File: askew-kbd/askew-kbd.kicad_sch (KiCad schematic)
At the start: 57 parts, among them J1 OLED, J2 MJ-4PP-9, SW1 SW_PUSH, SW10 SW_PUSH, SW11 SW_PUSH, SW12 SW_PUSH, SW13 SW_PUSH, SW14 SW_PUSH, SW15 SW_PUSH, SW16 SW_PUSH, SW17 SW_PUSH, SW18 SW_PUSH, SW19 SW_PUSH, SW2 SW_PUSH, SW20 SW_PUSH, SW21 SW_PUSH, SW22 SW_PUSH, SW3 SW_PUSH, SW4 SW_PUSH, SW5 SW_PUSH, SW6 SW_PUSH, SW7 SW_PUSH, SW8 SW_PUSH, SW9 SW_PUSH, U1 ProMicro

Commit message: choc_spacing
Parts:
- SW1, SW10, SW11, SW12, SW13, SW14, SW15, SW16, SW17, SW18, SW2, SW21, SW3, SW4, SW5, SW6, SW7, SW8, SW9: footprint fp:ChocV1_V2_Hotswap_reversed -> fp:ChocV1_V2_Hotswap_reversed_choc_spacing
- SW19, SW20, SW22: footprint fp:ChocV1_V2_Hotswap_reversed_15u -> fp:ChocV1_V2_Hotswap_reversed_15u_choc_spacing

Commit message: redo layout
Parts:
- D1, D10, D11, D12, D13, D14, D15, D16, D17, D18, D19, D2, D20, D21, D22, D3, D4, D5, D6, D7, D8, D9: footprint fp:D3_SMD -> kbd:D3_TH_SMD

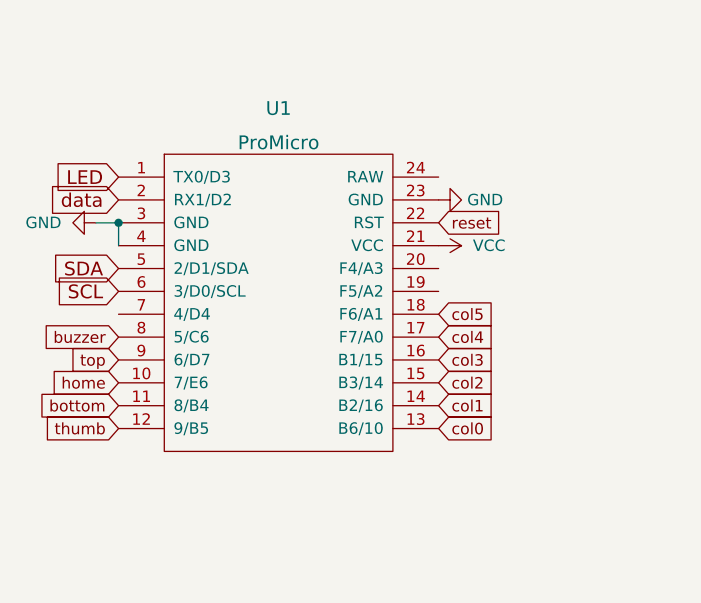
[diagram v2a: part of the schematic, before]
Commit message: basic routing
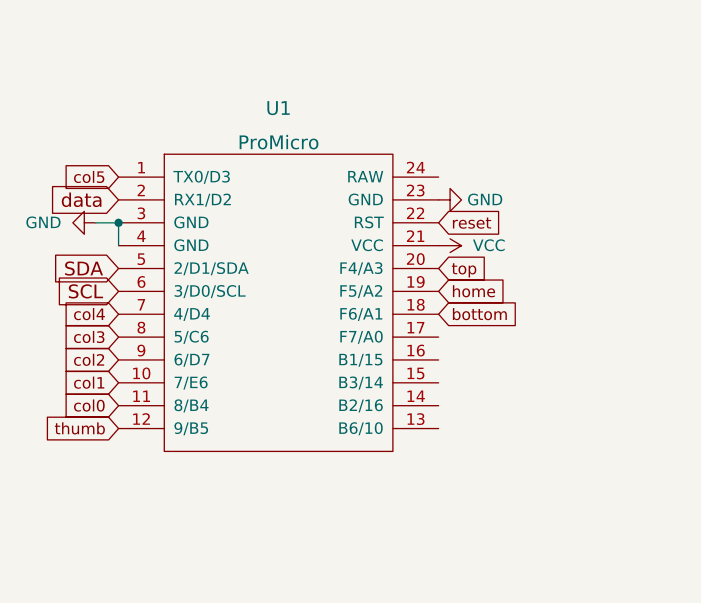
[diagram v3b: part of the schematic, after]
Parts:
- U1: footprint keyboard_reversible:ProMicro_unrouted -> fp:ProMicro_unrouted_type_c
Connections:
- net LED is gone; now on net col5: U1.1 (TX0/D3)
- net buzzer is gone; now on net col3: U1.8 (5/C6)
- net bottom: now also U1.18 (F6/A1); no longer U1.11 (8/B4)
- net col0: now also U1.11 (8/B4); no longer U1.13 (B6/10)
- net col1: now also U1.10 (7/E6); no longer U1.14 (B2/16)
- net col2: now also U1.9 (6/D7); no longer U1.15 (B3/14)
- net col3: no longer U1.16 (B1/15)
- net col4: now also U1.7 (4/D4); no longer U1.17 (F7/A0)
- net col5: no longer U1.18 (F6/A1)
- net home: now also U1.19 (F5/A2); no longer U1.10 (7/E6)
- net top: now also U1.20 (F4/A3); no longer U1.9 (6/D7)
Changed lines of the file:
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@@
     )
   )
-  (global_label "col0" (shape input) (at 91.44 74.93 0) (fields_autoplaced)
-    (effects (font (size 1.27 1.27)) (justify left))
-    (property "Intersheet References" "${INTERSHEET_REFS}" (id 0) (at 97.9655 74.8506 0)
-      (effects (font (size 1.27 1.27)) (justify left) hide)
+  (global_label "col0" (shape input) (at 55.88 72.39 180) (fields_autoplaced)
+    (effects (font (size 1.27 1.27)) (justify right))
+    (property "Intersheet References" "${INTERSHEET_REFS}" (id 0) (at 49.3545 72.4694 0)
+      (effects (font (size 1.27 1.27)) (justify right) hide)
     )
   )
@@
     )
   )
-  (global_label "bottom" (shape input) (at 55.88 72.39 180) (fields_autoplaced)
-    (effects (font (size 1.27 1.27)) (justify right))
-    (property "Intersheet References" "${INTERSHEET_REFS}" (id 0) (at 46.875 72.3106 0)
-      (effects (font (size 1.27 1.27)) (justify right) hide)
+  (global_label "bottom" (shape input) (at 91.44 62.23 0) (fields_autoplaced)
+    (effects (font (size 1.27 1.27)) (justify left))
+    (property "Intersheet References" "${INTERSHEET_REFS}" (id 0) (at 100.445 62.3094 0)
+      (effects (font (size 1.27 1.27)) (justify left) hide)
     )
   )
@@
     )
   )
-  (global_label "col5" (shape input) (at 91.44 62.23 0) (fields_autoplaced)
-    (effects (font (size 1.27 1.27)) (justify left))
-    (property "Intersheet References" "${INTERSHEET_REFS}" (id 0) (at 97.9655 62.1506 0)
-      (effects (font (size 1.27 1.27)) (justify left) hide)
+  (global_label "col5" (shape input) (at 55.88 46.99 180) (fields_autoplaced)
+    (effects (font (size 1.27 1.27)) (justify right))
+    (property "Intersheet References" "${INTERSHEET_REFS}" (id 0) (at 49.3545 47.0694 0)
+      (effects (font (size 1.27 1.27)) (justify right) hide)
     )
   )
@@
     )
   )
-  (global_label "LED" (shape input) (at 55.88 46.99 180) (fields_autoplaced)
-    (effects (font (size 1.524 1.524)) (justify right))
-    (property "Intersheet References" "${INTERSHEET_REFS}" (id 0) (at 264.795 142.875 0)
-      (effects (font (size 1.27 1.27)) hide)
-    )
-  )
-  (global_label "col3" (shape input) (at 91.44 67.31 0) (fields_autoplaced)
-    (effects (font (size 1.27 1.27)) (justify left))
-    (property "Intersheet References" "${INTERSHEET_REFS}" (id 0) (at 97.9655 67.2306 0)
-      (effects (font (size 1.27 1.27)) (justify left) hide)
+  (global_label "col3" (shape input) (at 55.88 64.77 180) (fields_autoplaced)
+    (effects (font (size 1.27 1.27)) (justify right))
+    (property "Intersheet References" "${INTERSHEET_REFS}" (id 0) (at 49.3545 64.8494 0)
+      (effects (font (size 1.27 1.27)) (justify right) hide)
     )
   )
@@
     )
   )
-  (global_label "col1" (shape input) (at 91.44 72.39 0) (fields_autoplaced)
-    (effects (font (size 1.27 1.27)) (justify left))
-    (property "Intersheet References" "${INTERSHEET_REFS}" (id 0) (at 97.9655 72.3106 0)
-      (effects (font (size 1.27 1.27)) (justify left) hide)
-    )
-  )
-  (global_label "buzzer" (shape input) (at 55.88 64.77 180) (fields_autoplaced)
+  (global_label "col1" (shape input) (at 55.88 69.85 180) (fields_autoplaced)
     (effects (font (size 1.27 1.27)) (justify right))
-    (property "Intersheet References" "${INTERSHEET_REFS}" (id 0) (at 47.2379 64.6906 0)
+    (property "Intersheet References" "${INTERSHEET_REFS}" (id 0) (at 49.3545 69.9294 0)
       (effects (font (size 1.27 1.27)) (justify right) hide)
     )
@@
     )
   )
-  (global_label "col2" (shape input) (at 91.44 69.85 0) (fields_autoplaced)
+  (global_label "col2" (shape input) (at 55.88 67.31 180) (fields_autoplaced)
+    (effects (font (size 1.27 1.27)) (justify right))
+    (property "Intersheet References" "${INTERSHEET_REFS}" (id 0) (at 49.3545 67.3894 0)
+      (effects (font (size 1.27 1.27)) (justify right) hide)
+    )
+  )
+  (global_label "home" (shape input) (at 91.44 59.69 0) (fields_autoplaced)
     (effects (font (size 1.27 1.27)) (justify left))
-    (property "Intersheet References" "${INTERSHEET_REFS}" (id 0) (at 97.9655 69.7706 0)
-      (effects (font (size 1.27 1.27)) (justify left) hide)
-    )
-  )
-  (global_label "home" (shape input) (at 55.88 69.85 180) (fields_autoplaced)
-    (effects (font (size 1.27 1.27)) (justify right))
-    (property "Intersheet References" "${INTERSHEET_REFS}" (id 0) (at 48.3869 69.7706 0)
-      (effects (font (size 1.27 1.27)) (justify right) hide)
+    (property "Intersheet References" "${INTERSHEET_REFS}" (id 0) (at 98.9331 59.7694 0)
+      (effects (font (size 1.27 1.27)) (justify left) hide)
     )
   )
@@
     )
   )
-  (global_label "top" (shape input) (at 55.88 67.31 180) (fields_autoplaced)
+  (global_label "top" (shape input) (at 91.44 57.15 0) (fields_autoplaced)
+    (effects (font (size 1.27 1.27)) (justify left))
+    (property "Intersheet References" "${INTERSHEET_REFS}" (id 0) (at 96.8769 57.2294 0)
+      (effects (font (size 1.27 1.27)) (justify left) hide)
+    )
+  )
+  (global_label "col4" (shape input) (at 55.88 62.23 180) (fields_autoplaced)
     (effects (font (size 1.27 1.27)) (justify right))
-    (property "Intersheet References" "${INTERSHEET_REFS}" (id 0) (at 50.4431 67.2306 0)
+    (property "Intersheet References" "${INTERSHEET_REFS}" (id 0) (at 49.3545 62.3094 0)
       (effects (font (size 1.27 1.27)) (justify right) hide)
-    )
-  )
-  (global_label "col4" (shape input) (at 91.44 64.77 0) (fields_autoplaced)
-    (effects (font (size 1.27 1.27)) (justify left))
-    (property "Intersheet References" "${INTERSHEET_REFS}" (id 0) (at 97.9655 64.6906 0)
-      (effects (font (size 1.27 1.27)) (justify left) hide)
     )
   )
@@
       (effects (font (size 1.524 1.524)))
     )
-    (property "Footprint" "keyboard_reversible:ProMicro_unrouted" (id 2) (at 76.2 87.63 0)
+    (property "Footprint" "fp:ProMicro_unrouted_type_c" (id 2) (at 76.2 87.63 0)
       (effects (font (size 1.524 1.524)) hide)
     )
@@
     )
     (path "/e8eb8608-eae3-4ab9-86a9-a5fe127a10fe"
-      (reference "U1") (unit 1) (value "ProMicro") (footprint "keyboard_reversible:ProMicro_unrouted")
-    )
-  )
+      (reference "U1") (unit 1) (value "ProMicro") (footprint "fp:ProMicro_unrouted_type_c")
+    )
+  )
